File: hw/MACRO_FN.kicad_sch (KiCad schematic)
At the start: 9 parts, among them J5 EXT

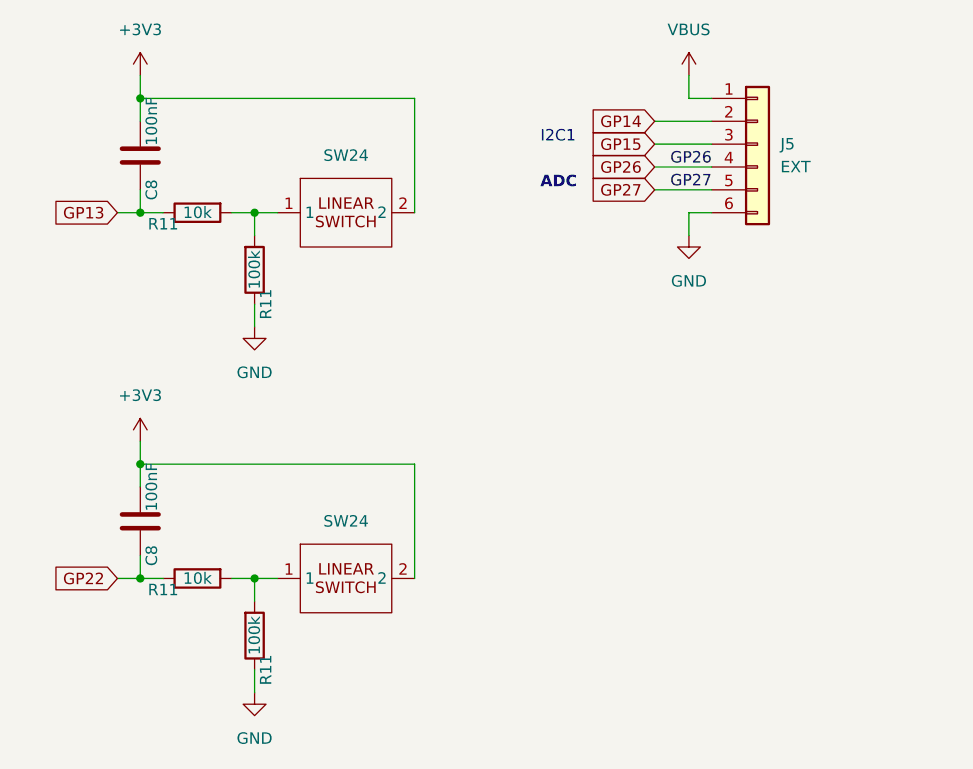
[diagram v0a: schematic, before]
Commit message: Schematic updated.
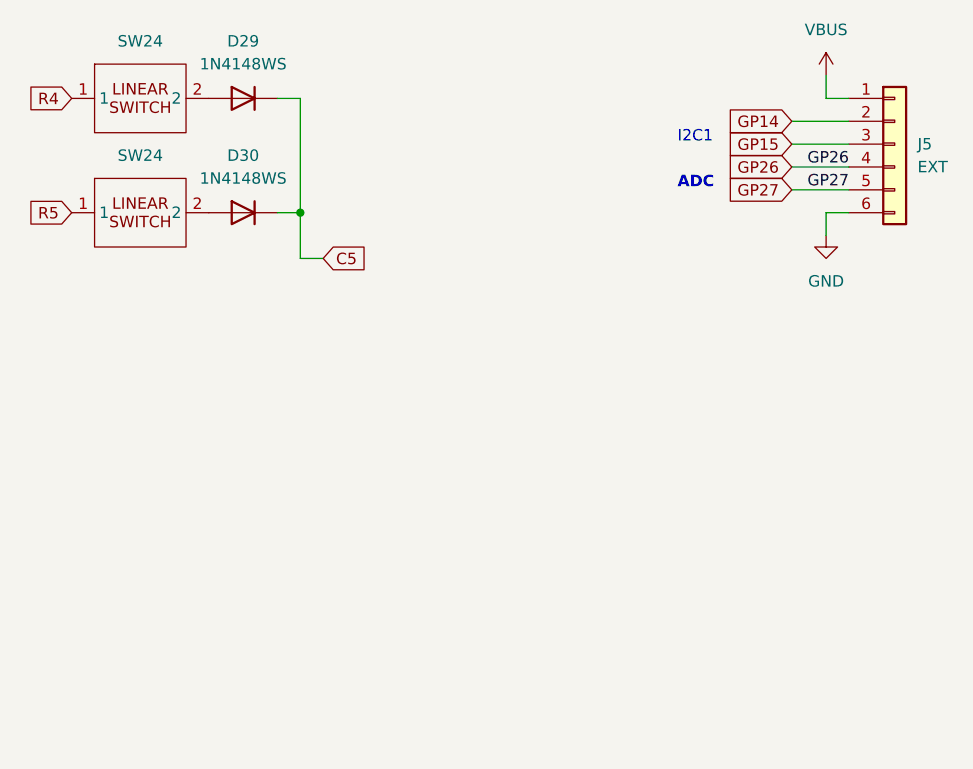
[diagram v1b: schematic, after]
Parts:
- removed C8 (x2): 100nF, Capacitor_SMD:C_0603_1608Metric, symbol Device:C
- removed R11 (x2): 100k, Resistor_SMD:R_0603_1608Metric, symbol Device:R
- removed R11 (x2): 10k, Resistor_SMD:R_0603_1608Metric, symbol Device:R
- removed SW24 (x2): ~, Keyboard_SW:Kailh_socket_MX_optional_reversible, symbol Keyboard:Linear_Switch
- added D29, D30: 1N4148WS, Diode_SMD:D_SOD-323, symbol Diode:1N4148WS
- added SW24 (x2): ~, Keyboard_SW:Kailh_socket_MX_optional_reversible, symbol Keyboard:Linear_Switch
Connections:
- new net: D29.2 (A), SW24.2
- new net: D30.2 (A), SW24.2
- new net C5: D29.1 (K), D30.1 (K)
- new net R4: SW24.1
- new net R5: SW24.1
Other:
- moved on the sheet: J5
